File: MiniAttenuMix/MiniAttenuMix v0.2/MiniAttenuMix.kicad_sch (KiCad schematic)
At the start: 38 parts, among them U1 TL072, U2 TL072, U3 TL074

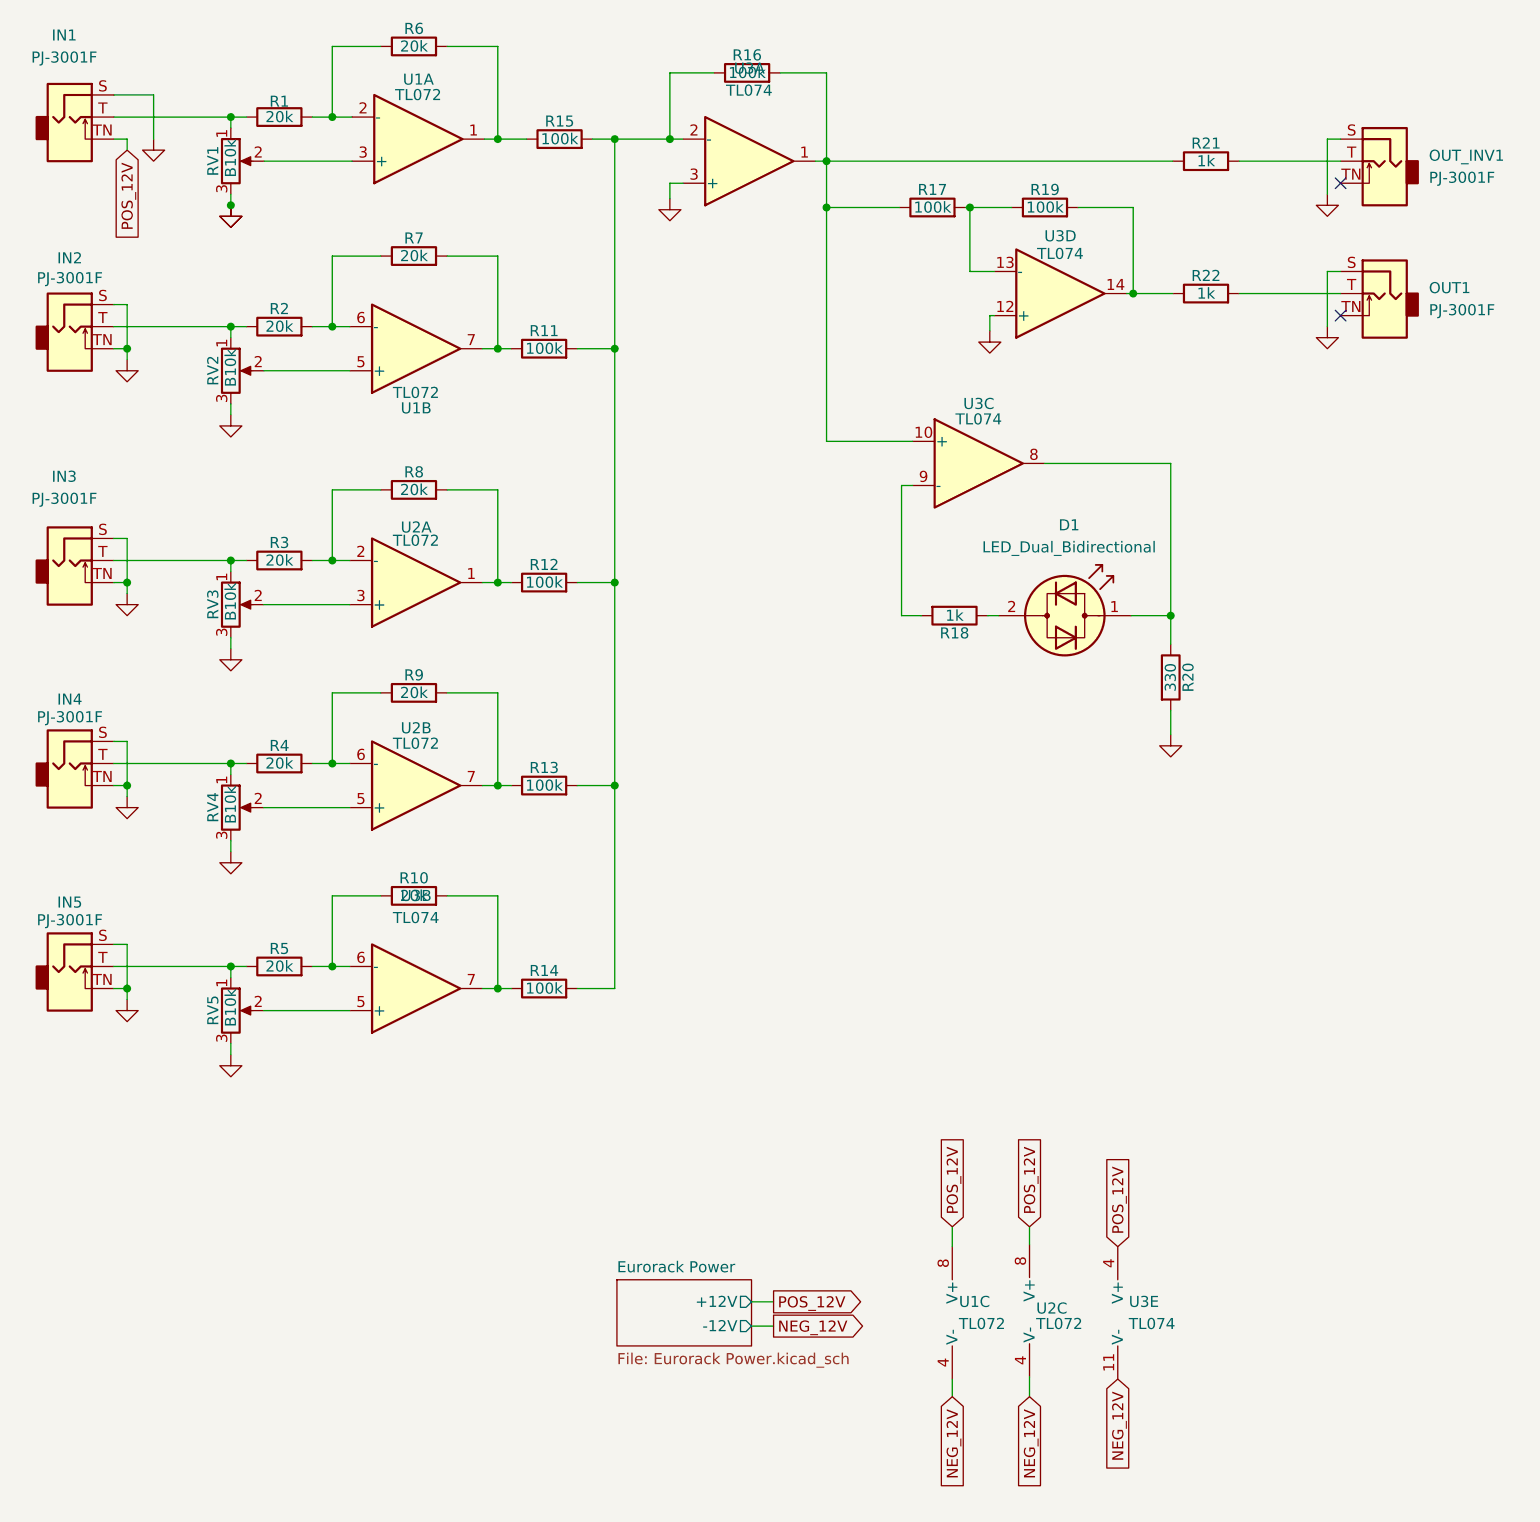
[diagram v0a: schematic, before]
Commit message: Added v0.2 gerbers
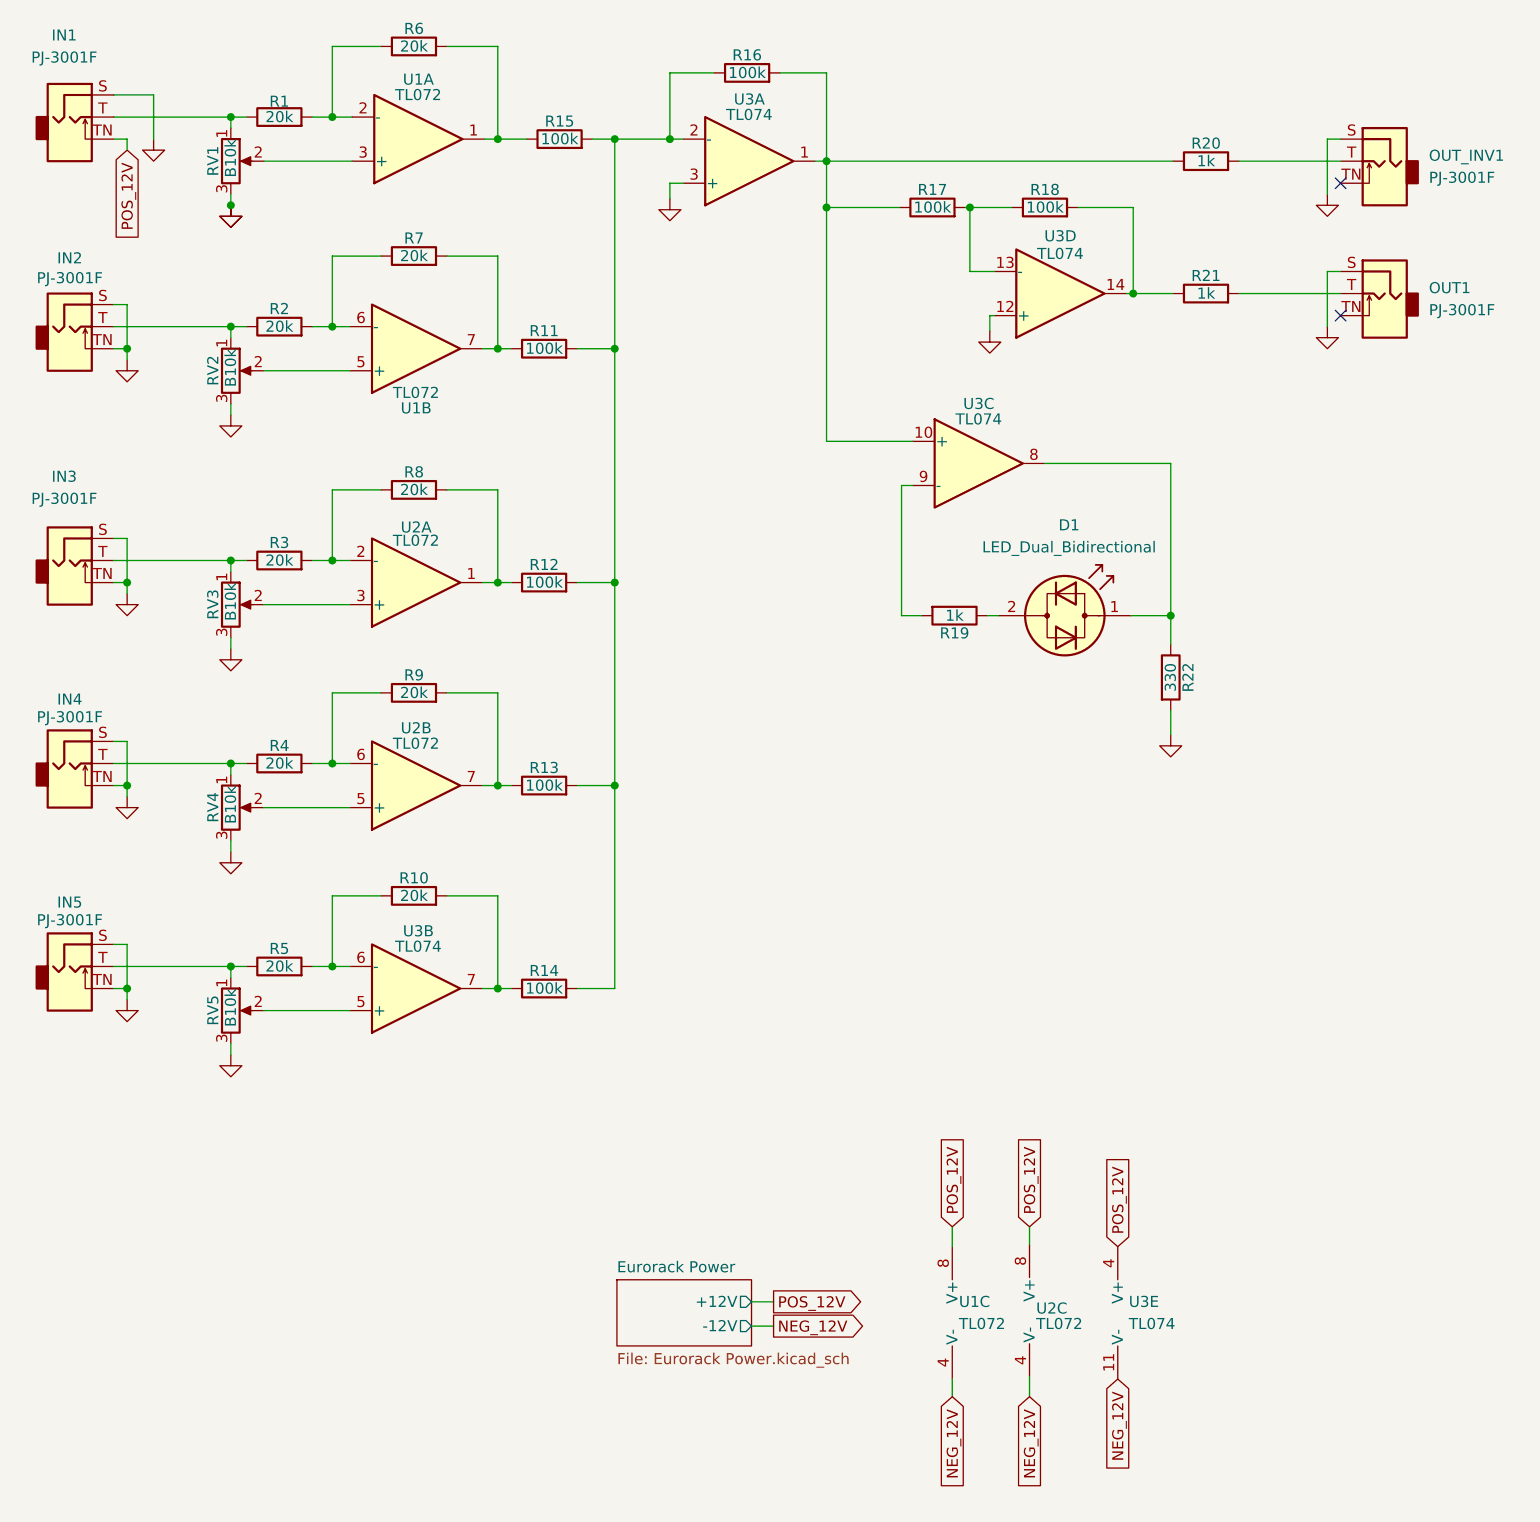
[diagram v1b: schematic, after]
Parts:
- renumbered R19 to R18, R18 to R19, R21 to R20, R22 to R21, R20 to R22
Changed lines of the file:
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@@
   (symbol (lib_id "Device:R") (at 147.32 92.202 270) (unit 1)
     (in_bom yes) (on_board yes)
-    (property "Reference" "R18" (id 0) (at 147.32 94.234 90))
+    (property "Reference" "R19" (id 0) (at 147.32 94.234 90))
     (property "Value" "1k" (id 1) (at 147.32 92.202 90))
     (property "Footprint" "Resistor_SMD:R_0603_1608Metric_Pad0.98x0.95mm_HandSolder" (id 2) (at 147.32 90.424 90)
@@
   (symbol (lib_id "Device:R") (at 157.734 45.212 90) (unit 1)
     (in_bom yes) (on_board yes)
-    (property "Reference" "R19" (id 0) (at 157.734 43.18 90))
+    (property "Reference" "R18" (id 0) (at 157.734 43.18 90))
     (property "Value" "100k" (id 1) (at 157.734 45.212 90))
     (property "Footprint" "Resistor_SMD:R_0603_1608Metric_Pad0.98x0.95mm_HandSolder" (id 2) (at 157.734 46.99 90)
@@
   (symbol (lib_id "Device:R") (at 176.276 55.118 90) (unit 1)
     (in_bom yes) (on_board yes)
-    (property "Reference" "R22" (id 0) (at 176.276 53.086 90))
+    (property "Reference" "R21" (id 0) (at 176.276 53.086 90))
     (property "Value" "1k" (id 1) (at 176.276 55.118 90))
     (property "Footprint" "Resistor_SMD:R_0603_1608Metric_Pad0.98x0.95mm_HandSolder" (id 2) (at 176.276 56.896 90)
@@
   )
   (symbol (lib_id "Amplifier_Operational:TL074") (at 123.698 39.878 0) (mirror x) (unit 1)
-    (in_bom yes) (on_board yes) (fields_autoplaced)
-    (property "Reference" "U3" (id 0) (at 123.698 29.21 0))
-    (property "Value" "TL074" (id 1) (at 123.698 31.75 0))
+    (in_bom yes) (on_board yes)
+    (property "Reference" "U3" (id 0) (at 123.698 32.766 0))
+    (property "Value" "TL074" (id 1) (at 123.698 34.544 0))
     (property "Footprint" "Package_SO:SOIC-14_3.9x8.7mm_P1.27mm" (id 2) (at 122.428 42.418 0)
       (effects (font (size 1.27 1.27)) hide)
@@
   (symbol (lib_id "Device:R") (at 172.212 99.314 0) (unit 1)
     (in_bom yes) (on_board yes)
-    (property "Reference" "R20" (id 0) (at 174.244 99.314 90))
+    (property "Reference" "R22" (id 0) (at 174.244 99.314 90))
     (property "Value" "330" (id 1) (at 172.212 99.314 90))
     (property "Footprint" "Resistor_SMD:R_0603_1608Metric_Pad0.98x0.95mm_HandSolder" (id 2) (at 170.434 99.314 90)
@@
   )
   (symbol (lib_id "Amplifier_Operational:TL074") (at 85.344 135.128 0) (mirror x) (unit 2)
-    (in_bom yes) (on_board yes) (fields_autoplaced)
-    (property "Reference" "U3" (id 0) (at 85.344 124.46 0))
-    (property "Value" "TL074" (id 1) (at 85.344 127 0))
+    (in_bom yes) (on_board yes)
+    (property "Reference" "U3" (id 0) (at 85.598 128.524 0))
+    (property "Value" "TL074" (id 1) (at 85.598 130.302 0))
     (property "Footprint" "Package_SO:SOIC-14_3.9x8.7mm_P1.27mm" (id 2) (at 84.074 137.668 0)
       (effects (font (size 1.27 1.27)) hide)
@@
   (symbol (lib_id "Device:R") (at 176.276 39.878 90) (unit 1)
     (in_bom yes) (on_board yes)
-    (property "Reference" "R21" (id 0) (at 176.276 37.846 90))
+    (property "Reference" "R20" (id 0) (at 176.276 37.846 90))
     (property "Value" "1k" (id 1) (at 176.276 39.878 90))
     (property "Footprint" "Resistor_SMD:R_0603_1608Metric_Pad0.98x0.95mm_HandSolder" (id 2) (at 176.276 41.656 90)
@@
   )
   (symbol_instances
-    (path "/6ca3117d-41e9-4e67-b1ed-864340ef5fb2/7855a11f-00a8-40e9-8791-ef424d300ca8"
-      (reference "#FLG01") (unit 1) (value "PWR_FLAG") (footprint "")
+    (path "/6ca3117d-41e9-4e67-b1ed-864340ef5fb2/266e0162-9a8c-4352-b329-043c3b3fcd60"
+      (reference "#FLG0101") (unit 1) (value "PWR_FLAG") (footprint "")
+    )
+    (path "/6ca3117d-41e9-4e67-b1ed-864340ef5fb2/856079e6-cb8d-4e4a-8323-4bd43d76057e"
+      (reference "#FLG0102") (unit 1) (value "PWR_FLAG") (footprint "")
+    )
+    (path "/6ca3117d-41e9-4e67-b1ed-864340ef5fb2/ed941bee-6953-4bf2-9fb3-9202ad39e9b3"
+      (reference "#FLG0103") (unit 1) (value "PWR_FLAG") (footprint "")
     )
     (path "/e9d916b3-b487-4293-820b-6be0daabdae8"
@@
       (reference "#PWR019") (unit 1) (value "-12V") (footprint "")
     )
-    (path "/6ca3117d-41e9-4e67-b1ed-864340ef5fb2/f0c47c54-c94f-49c4-ac4e-3132ae4fcc66"
+    (path "/6ca3117d-41e9-4e67-b1ed-864340ef5fb2/3249749f-33a7-4c50-b089-7eda4e31bb87"
       (reference "C1") (unit 1) (value "22uF") (footprint "Capacitor_SMD:C_0805_2012Metric_Pad1.18x1.45mm_HandSolder")
     )
-    (path "/6ca3117d-41e9-4e67-b1ed-864340ef5fb2/56692e65-dc73-41d1-ad12-71cca6b2431a"
+    (path "/6ca3117d-41e9-4e67-b1ed-864340ef5fb2/fd6925d6-e461-4f37-ac76-35badc9263d9"
       (reference "C2") (unit 1) (value "22uF") (footprint "Capacitor_SMD:C_0805_2012Metric_Pad1.18x1.45mm_HandSolder")
     )
@@
       (reference "R17") (unit 1) (value "100k") (footprint "Resistor_SMD:R_0603_1608Metric_Pad0.98x0.95mm_HandSolder")
     )
+    (path "/5d37291e-4f28-4ec8-8e19-a9bdf88181d5"
+      (reference "R18") (unit 1) (value "100k") (footprint "Resistor_SMD:R_0603_1608Metric_Pad0.98x0.95mm_HandSolder")
+    )
     (path "/0b1909f4-69bf-4c76-9b29-d55df5dae511"
-      (reference "R18") (unit 1) (value "1k") (footprint "Resistor_SMD:R_0603_1608Metric_Pad0.98x0.95mm_HandSolder")
-    )
-    (path "/5d37291e-4f28-4ec8-8e19-a9bdf88181d5"
-      (reference "R19") (unit 1) (value "100k") (footprint "Resistor_SMD:R_0603_1608Metric_Pad0.98x0.95mm_HandSolder")
+      (reference "R19") (unit 1) (value "1k") (footprint "Resistor_SMD:R_0603_1608Metric_Pad0.98x0.95mm_HandSolder")
+    )
+    (path "/e663cc4e-e689-4acf-801f-a2158067730a"
+      (reference "R20") (unit 1) (value "1k") (footprint "Resistor_SMD:R_0603_1608Metric_Pad0.98x0.95mm_HandSolder")
+    )
+    (path "/72e99c7d-55ab-410a-b5f7-1440e9934549"
+      (reference "R21") (unit 1) (value "1k") (footprint "Resistor_SMD:R_0603_1608Metric_Pad0.98x0.95mm_HandSolder")
     )
     (path "/8b83dc9a-cab6-4341-ac90-b3ebfd256dba"
-      (reference "R20") (unit 1) (value "330") (footprint "Resistor_SMD:R_0603_1608Metric_Pad0.98x0.95mm_HandSolder")
-    )
-    (path "/e663cc4e-e689-4acf-801f-a2158067730a"
-      (reference "R21") (unit 1) (value "1k") (footprint "Resistor_SMD:R_0603_1608Metric_Pad0.98x0.95mm_HandSolder")
-    )
-    (path "/72e99c7d-55ab-410a-b5f7-1440e9934549"
-      (reference "R22") (unit 1) (value "1k") (footprint "Resistor_SMD:R_0603_1608Metric_Pad0.98x0.95mm_HandSolder")
+      (reference "R22") (unit 1) (value "330") (footprint "Resistor_SMD:R_0603_1608Metric_Pad0.98x0.95mm_HandSolder")
     )
     (path "/f264f21d-5749-43d9-8e7e-3b86ad9cd4bf"
